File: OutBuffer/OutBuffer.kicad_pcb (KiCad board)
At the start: 2 copper layers, 60 x 37 mm, 84 parts, among them J1 JST_PH_S6B-PH-K, J2 JST_PH_B3B-PH-K, J3 RND 205-00698, J4 RND 205-00698, J5 JST_PH_S3B-PH-K, J6 JST_PH_S3B-PH-K, U1 AD797, U2 AD797, U3 AD797, U4 AD797, U5 AD797, U6 AD797

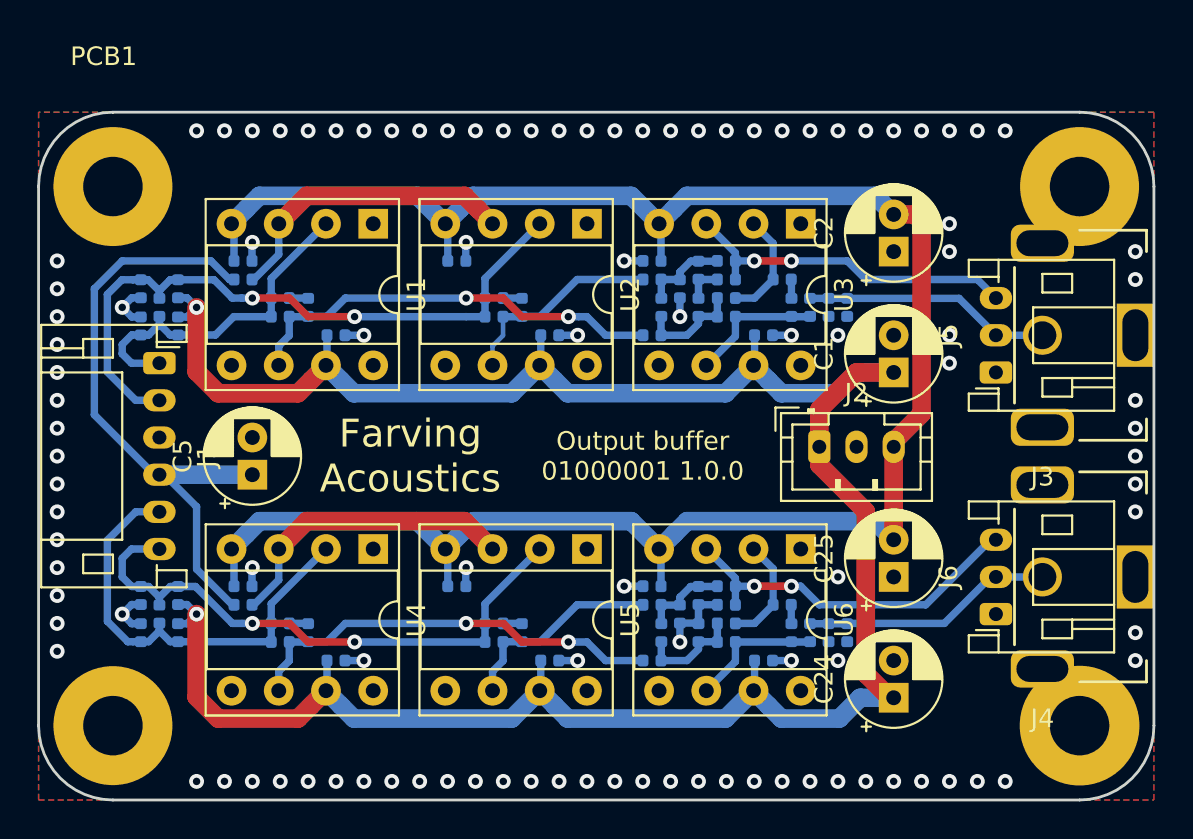
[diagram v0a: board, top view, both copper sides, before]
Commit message: Release 1.0.0
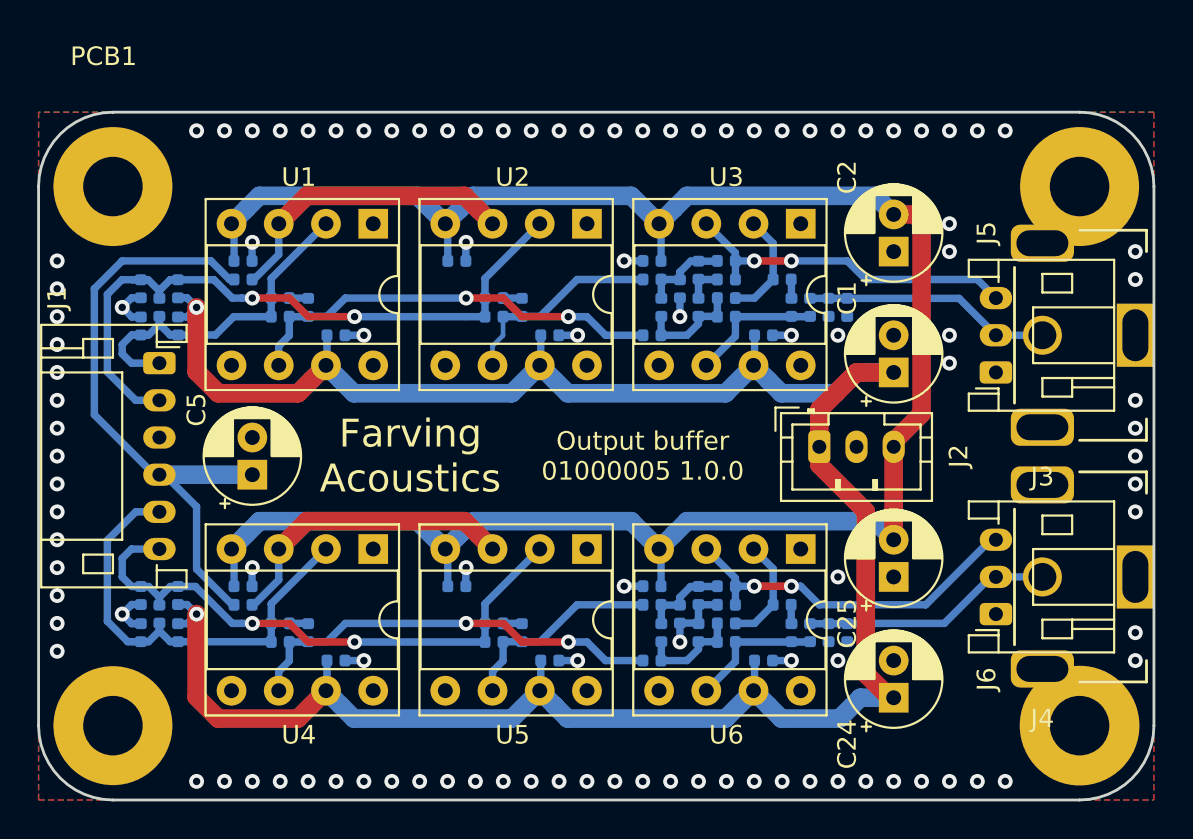
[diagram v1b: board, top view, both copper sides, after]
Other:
- board text added: "Output buffer 01000005 1.0.0"
- board text removed: "Output buffer 01000001 1.0.0"
